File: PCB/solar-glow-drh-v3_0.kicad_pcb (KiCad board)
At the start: 2 copper layers, 50.8 x 88.9 mm, 62 parts, among them J1 UPDI hdr, Q1 BCP5316MTWG, SW2 LED master, U1 AVR64DD28 (VQFN28), U2 ALD910025SALI, U3 ADXL367, U4 TLV3011BIDBVR, U5 NT3H2211, U6 TPS22918

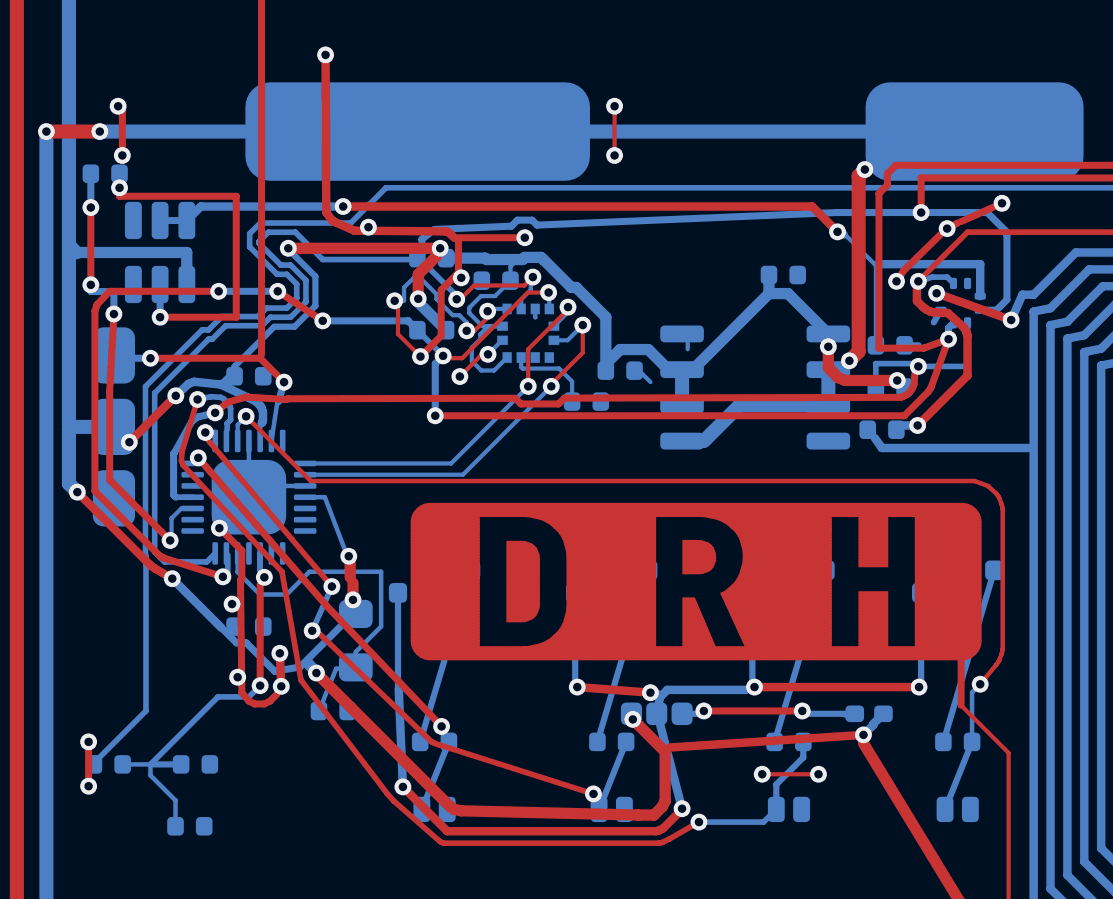
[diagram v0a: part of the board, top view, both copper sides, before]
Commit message: Add files via upload
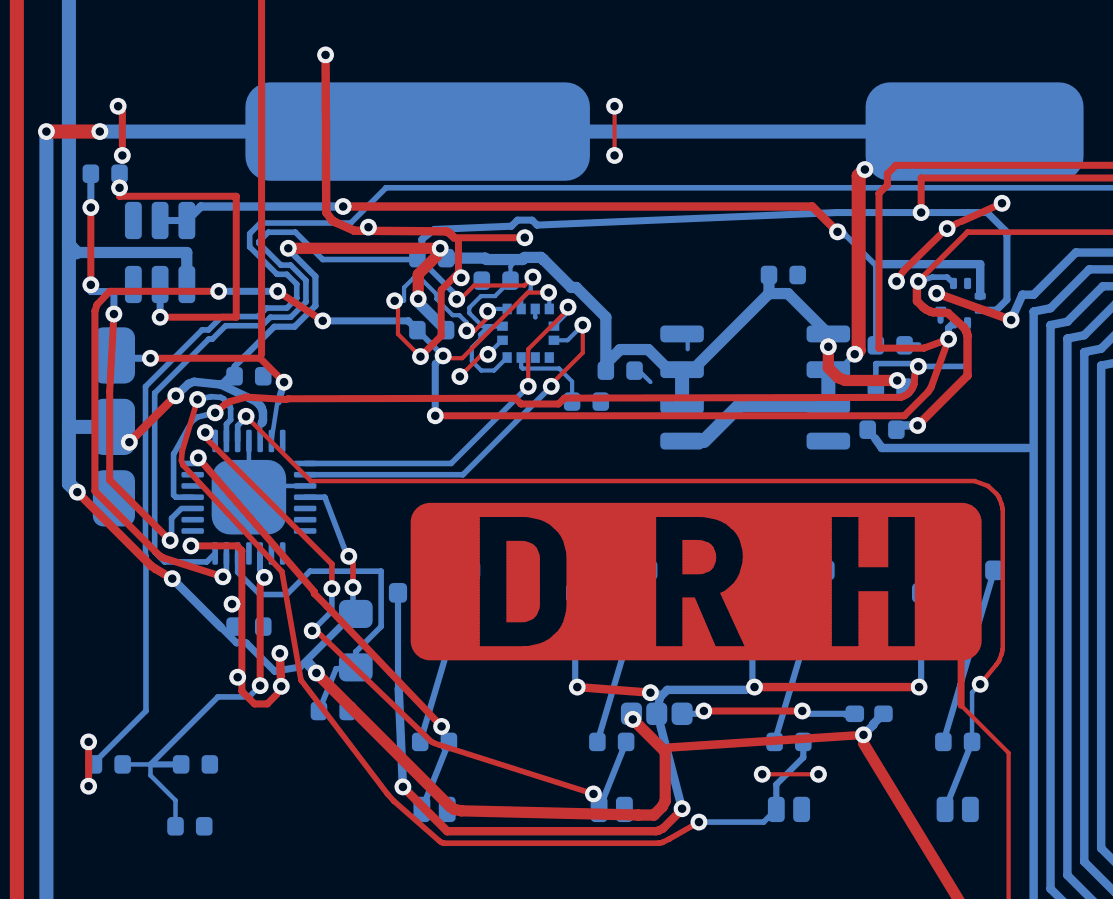
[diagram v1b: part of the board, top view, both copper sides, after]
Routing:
- net VS: track 292.5 -> 293.2 mm
- net GND: track 127.0 -> 127.6 mm
